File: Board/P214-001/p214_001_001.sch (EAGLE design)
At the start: 24 parts, among them IC1 74LS07N

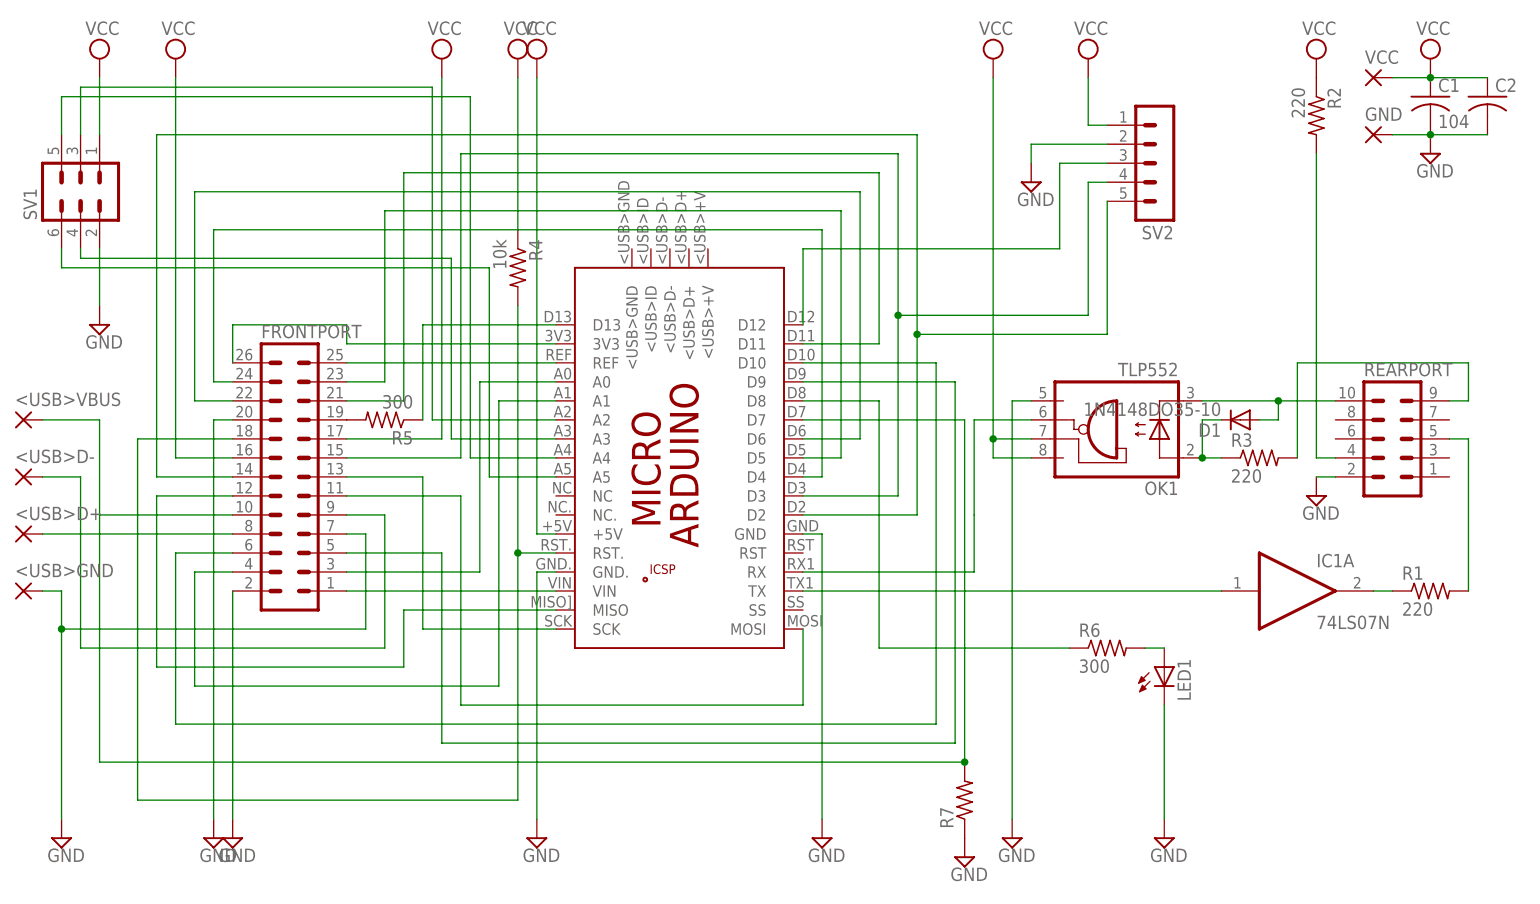
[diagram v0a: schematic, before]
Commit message: new design.
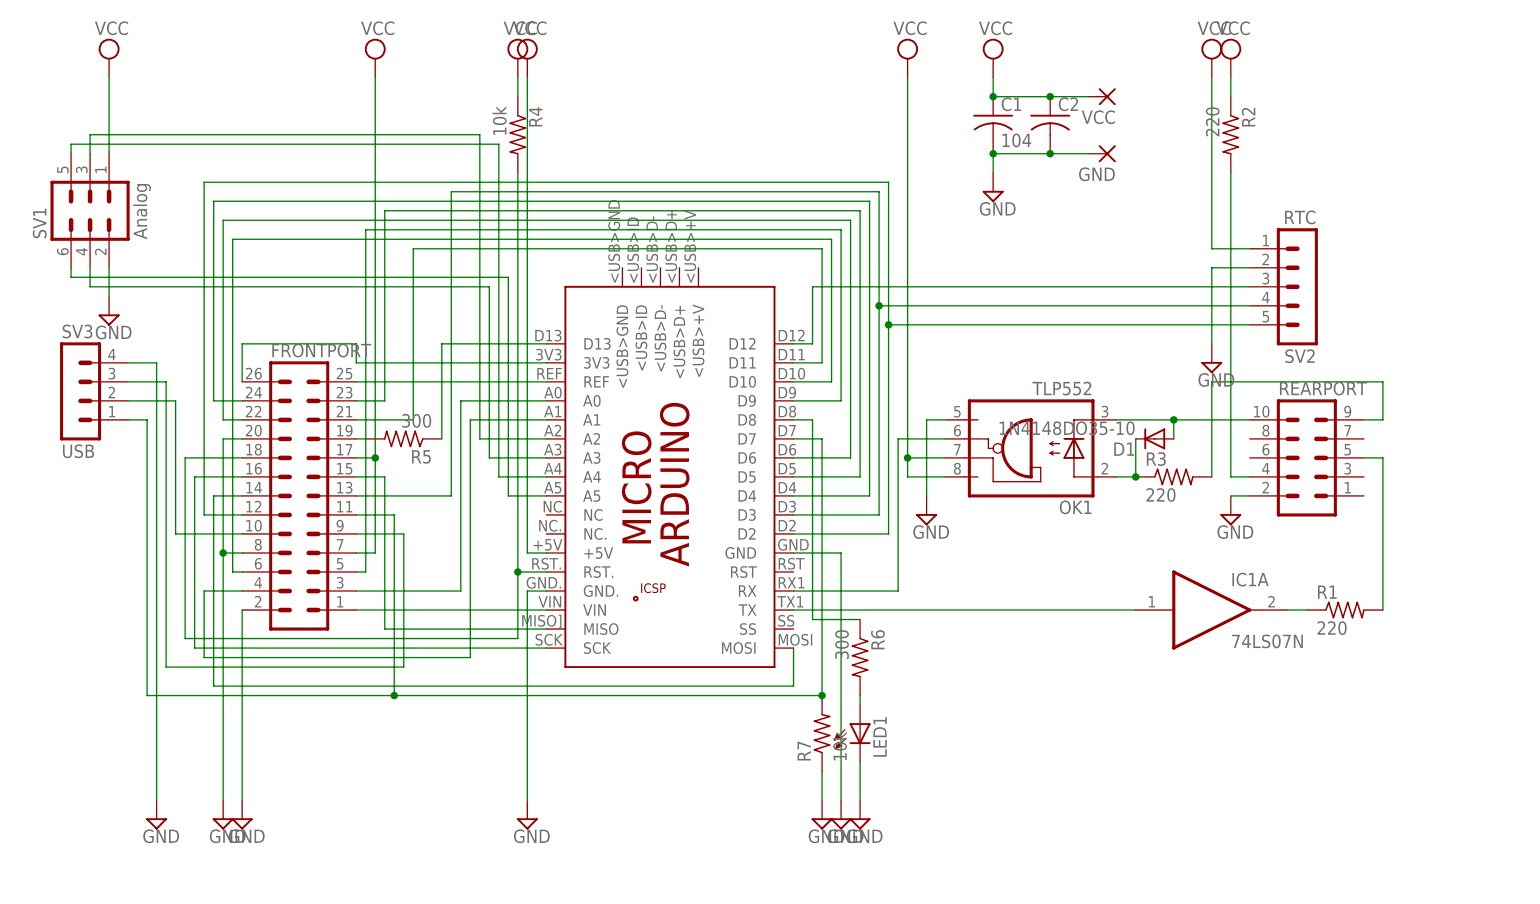
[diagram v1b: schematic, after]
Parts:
- removed <USB>D+, <USB>D-, <USB>GND, <USB>VBUS: (no value), wirepad:1,6/0,9
- added SV3: USB, con-lstb:MA04-1
- R7: value (none) -> 10k
- SV1: value (none) -> Analog
- SV2: value (none) -> RTC
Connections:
- removed net N$25: <USB>VBUS.P, FRONTPORT.10, PCB1.D7, R7.2
- new net N$39: FRONTPORT.10, SV3.2
- net GND: now also FRONTPORT.8, SV3.4; no longer <USB>GND.P, FRONTPORT.7
- net N$14: now also FRONTPORT.14; no longer FRONTPORT.11
- net N$15: now also FRONTPORT.15; no longer FRONTPORT.12
- net N$16: now also FRONTPORT.16; no longer FRONTPORT.13
- net N$17: now also FRONTPORT.12; no longer FRONTPORT.14
- net N$18: now also FRONTPORT.13; no longer FRONTPORT.15
- net N$22: now also SV3.3; no longer <USB>D-.P
- net N$24: now also FRONTPORT.11, PCB1.D7, R7.2, SV3.1; no longer <USB>D+.P, FRONTPORT.8
- net VCC: now also FRONTPORT.7; no longer FRONTPORT.16
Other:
- moved on the sheet: C1, C2, D1, FRONTPORT, GND, IC1A, LED1, OK1, R1, R2, R3, R4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
